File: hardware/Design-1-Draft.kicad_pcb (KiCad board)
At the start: 2 copper layers, 32 parts, among them J1 Barrel_Jack_Switch, M1 WATERPUMP-1, M2 WATERPUMP-2, Q1 IRLZ44N, Q2 IRLZ44N, SW1 Button, U3 ADS1115IDGS, U5 Tang_Nano_9K

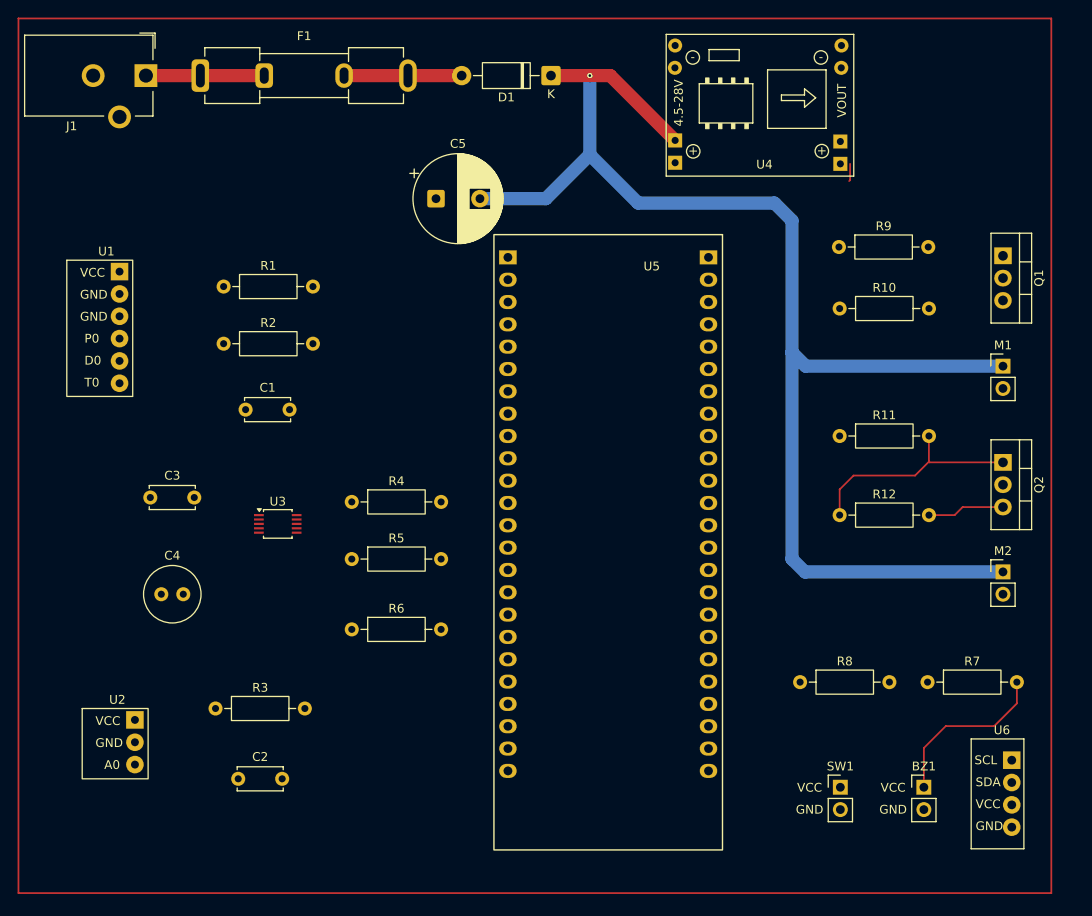
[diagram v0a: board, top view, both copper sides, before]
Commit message: updated schematic and pcb
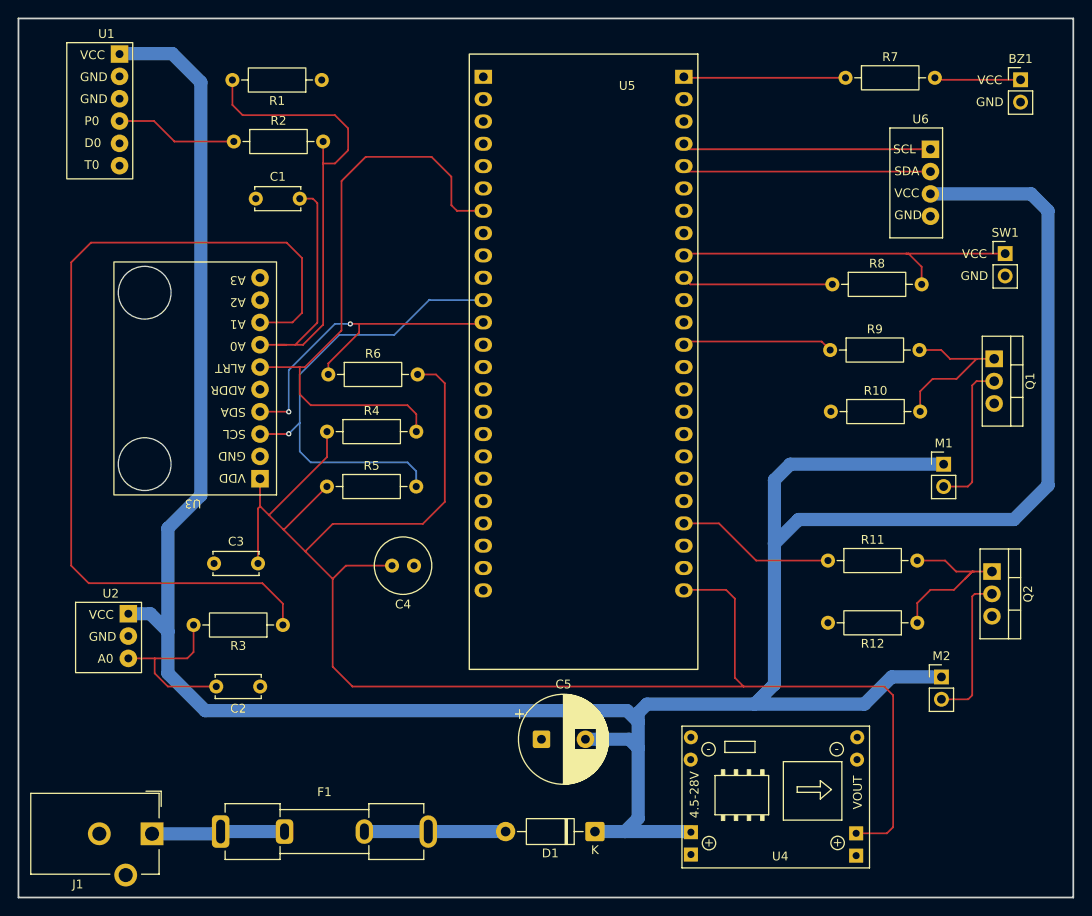
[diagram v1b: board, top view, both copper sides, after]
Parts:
- U3: footprint Package_SO:TSSOP-10_3x3mm_P0.5mm -> 1_CustomFootprints:ADS1115
- moved J1 86.3 mm to (81.7, 126.8)
- moved D1 86.1 mm to (132.1, 126.5)
- moved F1 86.0 mm to (89.5, 126.5)
- moved BZ1 81.2 mm to (180.5, 41.0)
- moved U4 78.7 mm to (153.2, 122.0)
- moved U6 70.1 mm to (168.8, 52.7)
- moved R7 69.4 mm to (160.6, 40.8)
- moved SW1 63.5 mm to (178.8, 60.8)
- moved C5 62.7 mm to (126.0, 116.0)
- moved R8 45.4 mm to (159.1, 64.2)
- moved R6 29.1 mm to (101.8, 74.5)
- moved C4 28.9 mm to (111.5, 96.2), turned to 180 degrees
- moved R1 26.0 mm to (101.0, 41.0), turned to 180 degrees
- moved U1 24.8 mm to (76.0, 44.2)
- moved C1 24.0 mm to (93.5, 54.5)
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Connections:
- R11 pad 1: Net-(U5-70_IOT41B) -> Net-(U5-31_IOB15A)
- R8 pad 1: Net-(U5-72_IOT39B) -> Net-(U5-77_IOT37A)
- R8 pad 2: Net-(U5-73_IOT39A) -> Net-(U5-79_IOT12B_1V8)
- R9 pad 1: Net-(U5-71_IOT41A) -> Net-(U5-74_IOT38B)
- SW1 pad 1: Net-(U5-73_IOT39A) -> Net-(U5-79_IOT12B_1V8)
- U5 pad 28: unconnected-(U5-31_IOB15A-Pad28) -> Net-(U5-31_IOB15A)
- U5 pad 32: Net-(U5-70_IOT41B) -> unconnected-(U5-70_IOT41B-Pad32)
- U5 pad 33: Net-(U5-71_IOT41A) -> unconnected-(U5-71_IOT41A-Pad33)
- U5 pad 34: Net-(U5-72_IOT39B) -> unconnected-(U5-72_IOT39B-Pad34)
- U5 pad 35: Net-(U5-73_IOT39A) -> unconnected-(U5-73_IOT39A-Pad35)
- U5 pad 36: unconnected-(U5-74_IOT38B-Pad36) -> Net-(U5-74_IOT38B)
- U5 pad 39: unconnected-(U5-77_IOT37A-Pad39) -> Net-(U5-77_IOT37A)
- U5 pad 40: unconnected-(U5-79_IOT12B_1V8-Pad40) -> Net-(U5-79_IOT12B_1V8)
- U5 pad 42: Net-(U5-81_IOT11B_1V8) -> unconnected-(U5-81_IOT11B_1V8-Pad42)
- U5 pad 43: Net-(U5-82_IOT11A_1V8) -> unconnected-(U5-82_IOT11A_1V8-Pad43)
- U5 pad 44: unconnected-(U5-83_IOT10B_1V8-Pad44) -> Net-(U5-83_IOT10B_1V8)
- U5 pad 45: unconnected-(U5-84_IOT10A_1V8-Pad45) -> Net-(U5-84_IOT10A_1V8)
- U6 pad 1: Net-(U5-82_IOT11A_1V8) -> Net-(U5-84_IOT10A_1V8)
- U6 pad 2: Net-(U5-81_IOT11B_1V8) -> Net-(U5-83_IOT10B_1V8)
- U6 pad 3: Net-(U3-VDD) -> Net-(D1-K)
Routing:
- net Net-(U3-VDD): track 0.00 -> 194.5 mm
- net Net-(D1-K): track 154.7 -> 334.0 mm, vias 1 -> 0
- net Net-(U3-AIN1): track 0.00 -> 102.2 mm
- net Net-(U3-AIN0): track 0.00 -> 72.3 mm
- net Net-(U3-ALERT/RDY): track 0.00 -> 69.0 mm
- net Net-(U3-SCL): track 0.00 -> 54.2 mm, vias 0 -> 1
- net Net-(U5-79_IOT12B_1V8): track 0.00 -> 41.4 mm
- net Net-(U3-SDA): track 0.00 -> 39.6 mm, vias 0 -> 2
- net Net-(U5-84_IOT10A_1V8): track 0.00 -> 28.3 mm
- net Net-(U5-83_IOT10B_1V8): track 0.00 -> 28.3 mm
- net Net-(U2-A0): track 0.00 -> 20.1 mm
- net Net-(Q1-G): track 0.00 -> 19.2 mm
- net Net-(U5-63_IOR5A): track 0.00 -> 18.4 mm
- net Net-(U5-31_IOB15A): track 0.00 -> 18.1 mm
- net Net-(M2--): track 0.00 -> 17.3 mm
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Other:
- board outline added: 120 x 100 mm
